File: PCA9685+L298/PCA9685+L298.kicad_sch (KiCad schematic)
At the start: 95 parts, among them J1 TERMBLOCK_1X2, J10 TERMBLOCK_1X2, J11 TERMBLOCK_1X2, J13 Conn_01x04, J4 TERMBLOCK_1X2, J5 TERMBLOCK_1X2, J7 QWIIC_RIGHT_ANGLE, J7 TERMBLOCK_1X2, J8 TERMBLOCK_1X2, Q1 AOD417, U1 PCA9685, U2 L298HN, U3 L298HN, U4 L298HN, U5 ADS1115IDGS, U6 ADS1115IDGS, U7 ADS1115IDGS, U8 L7805

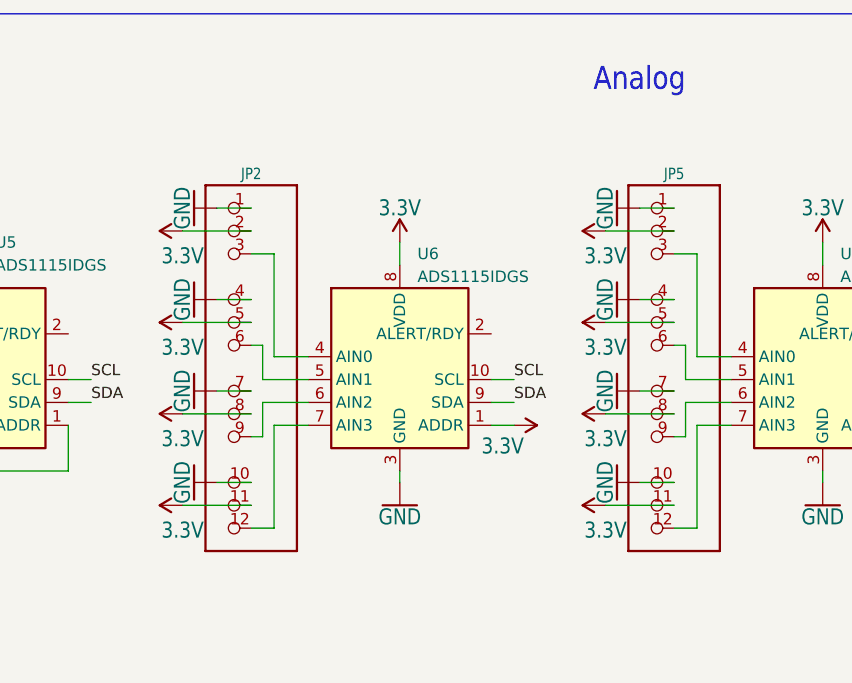
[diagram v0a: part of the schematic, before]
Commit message: rev 0
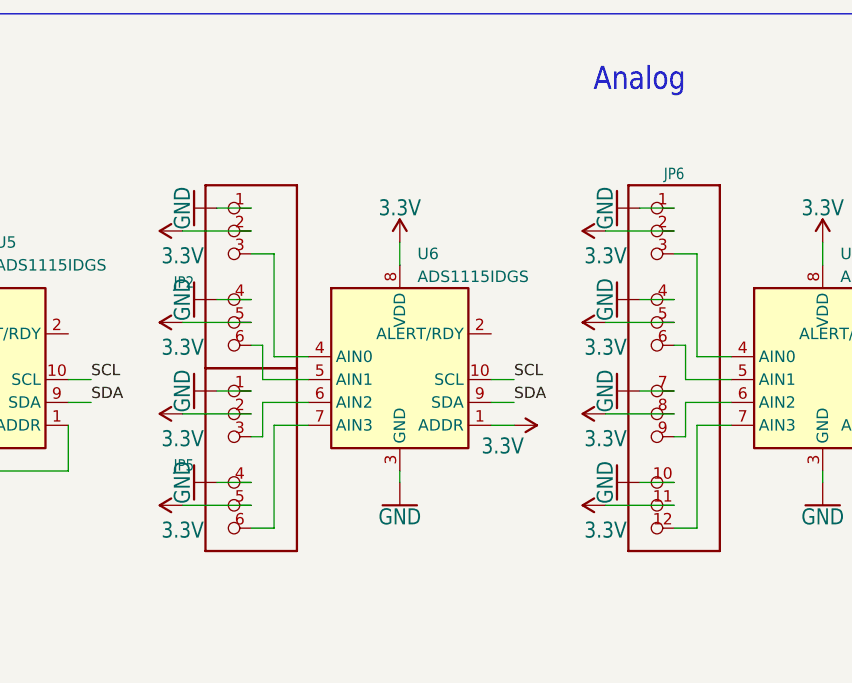
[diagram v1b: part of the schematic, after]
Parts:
- removed JP2, JP5: ~, Adafruit PCA9685 rev C:3X04, symbol Adafruit PCA9685 rev C-eagle-import:HEADER-3X04
- added JP2, JP5: ~, Adafruit PCA9685 rev C:3X02, symbol Adafruit PCA9685 rev C-eagle-import:HEADER-3X02
- added JP6: ~, Adafruit PCA9685 rev C:3X04, symbol Adafruit PCA9685 rev C-eagle-import:HEADER-3X04
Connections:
- net 3.3V: now also JP2.2, JP2.5, JP5.2, JP5.5, JP6.11, JP6.2, JP6.5, JP6.8
- net GND: now also JP2.1, JP2.4, JP5.1, JP5.4, JP6.1, JP6.10, JP6.4, JP6.7
- net at U7.4 (AIN0): now also JP6.3
- net at U7.5 (AIN1): now also JP6.6
- net at U7.6 (AIN2): now also JP6.9
- net at U7.7 (AIN3): now also JP6.12
- net at U6.4 (AIN0): now also JP2.3
- net at U6.5 (AIN1): now also JP2.6
- net at U6.6 (AIN2): now also JP5.3
- net at U6.7 (AIN3): now also JP5.6

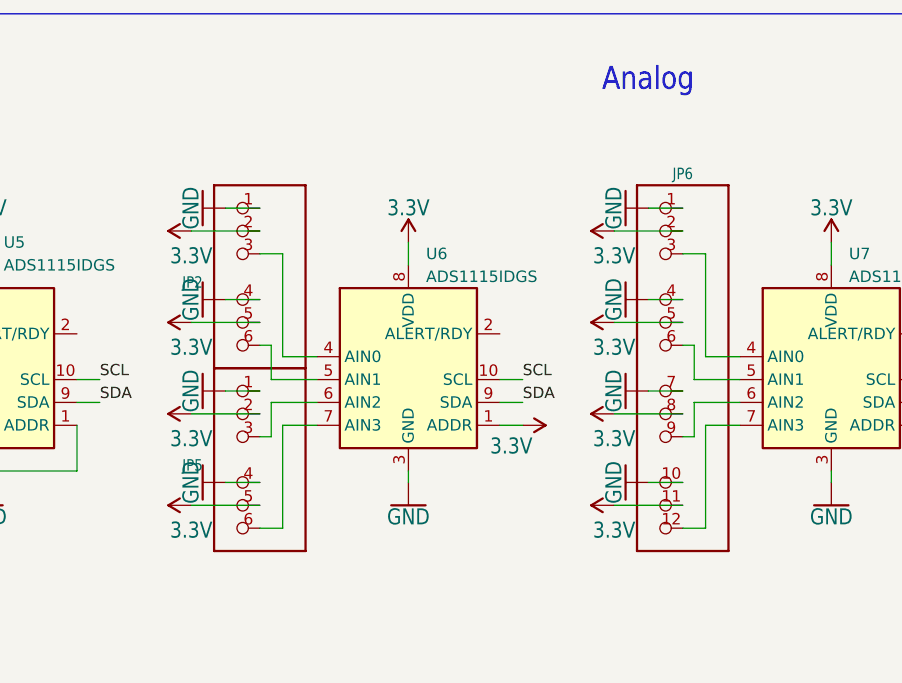
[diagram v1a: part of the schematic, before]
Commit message: 23.04.23
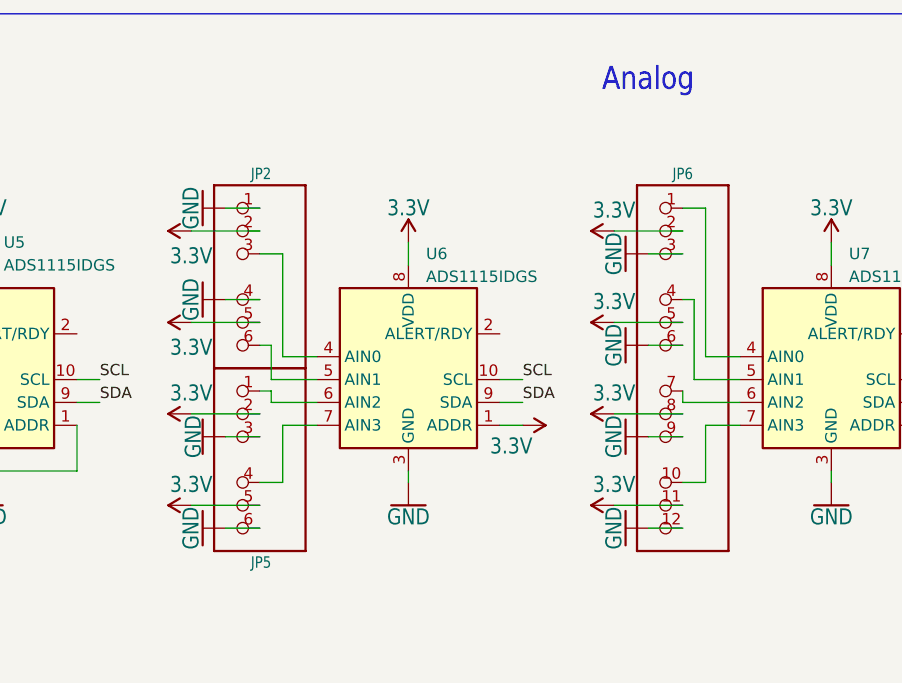
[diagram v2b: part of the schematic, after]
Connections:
- net GND: now also JP5.3, JP5.6, JP6.12, JP6.3, JP6.6, JP6.9; no longer JP5.1, JP5.4, JP6.1, JP6.10, JP6.4, JP6.7
- net at U7.4 (AIN0): now also JP6.1; no longer JP6.3
- net at U7.5 (AIN1): now also JP6.4; no longer JP6.6
- net at U7.6 (AIN2): now also JP6.7; no longer JP6.9
- net at U7.7 (AIN3): now also JP6.10; no longer JP6.12
- net at U6.6 (AIN2): now also JP5.1; no longer JP5.3
- net at U6.7 (AIN3): now also JP5.4; no longer JP5.6
